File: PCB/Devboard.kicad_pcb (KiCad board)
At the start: 2 copper layers, 133.4 x 151 mm, 602 parts, among them J1 HR911105A_C12074, Q1 IPB180P04P4L-02, Q2 IPB180P04P4L-02, SW1 SW_Push, U1 TVS2201DRBR, U10 TPS62822DLCR, U11 TPS62823DLCR, U12 TPS548A20RVER, U13 TPS7A4700RGWR, U14 TPS3700DSET, U15 TPS54824RNVR, U16 TPS54824RNVR, U17 TPS7A4700RGWR, U18 DW06, U19 TPS61088RHLR, U2 TPD6S300ARUKR, U20 TPS54824RNVR, U21 LM66100DCK, U22 TPS7A4700RGWR, U23 TPS7A4700RGWR, U24 TPS259470ARPWR, U25 TPS54824RNVR, U26 xczu4evfbvb900pkg, U27 RS3112-1.25XSF3, U28 MT25QU256ABA8ESF-0SIT TR, U29 FEMDNN032G-A3A55, U3 STUSB4500QTR, U30 TXS02612RTWR, U31 DP83867IRRGZR, U32 USB3320C-EZK-TR, U34 CP2102N-Axx-xQFN24, U35 TXB0108PW, U36 TCA9548APWR, U37 PCA9306, U38 TPD4E05U06DQA, U4 TPS2121RUXR, U5 TPS259470ARPWR, U6 BQ25895RTWR, U7 BQ27441DRZR-G1A, U8 TPS62130RGTR, U9 XT60, Y1 25 MHz, Y2 25 MHz

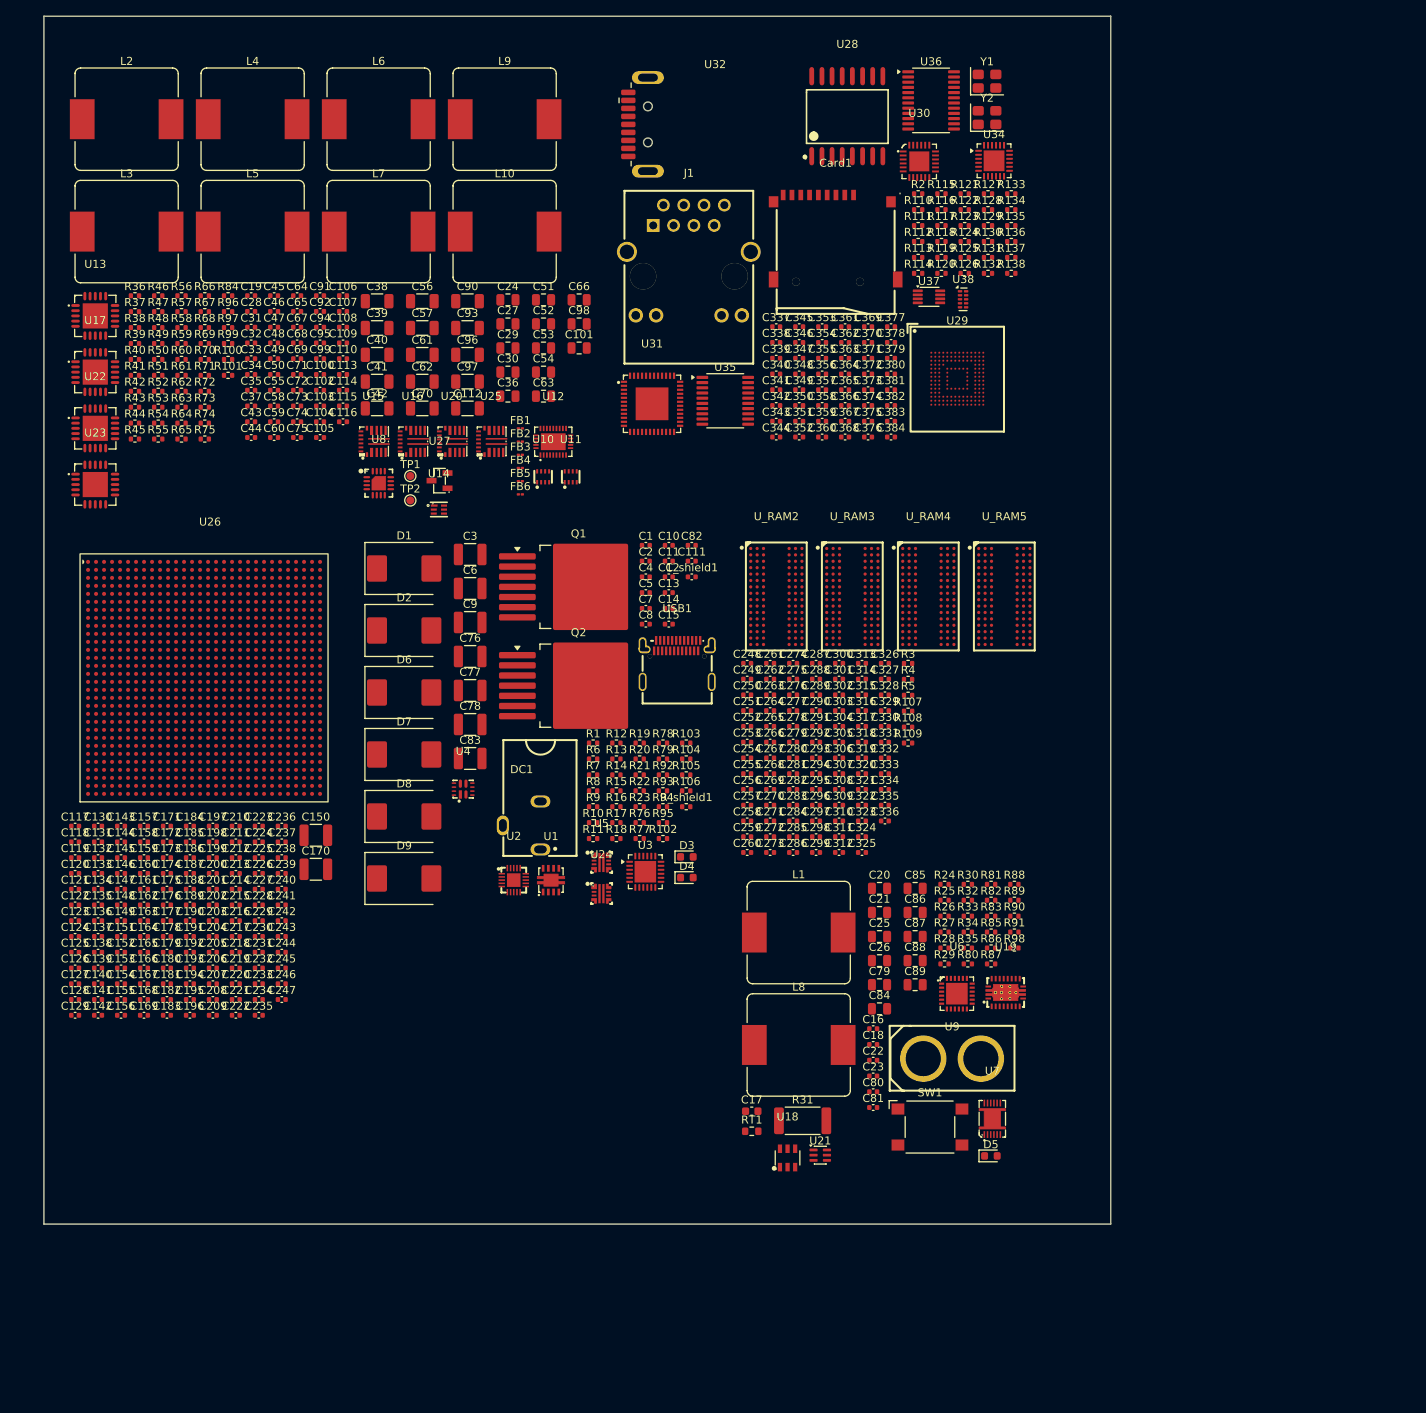
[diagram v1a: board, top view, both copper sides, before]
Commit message: feat: Section 4 Done
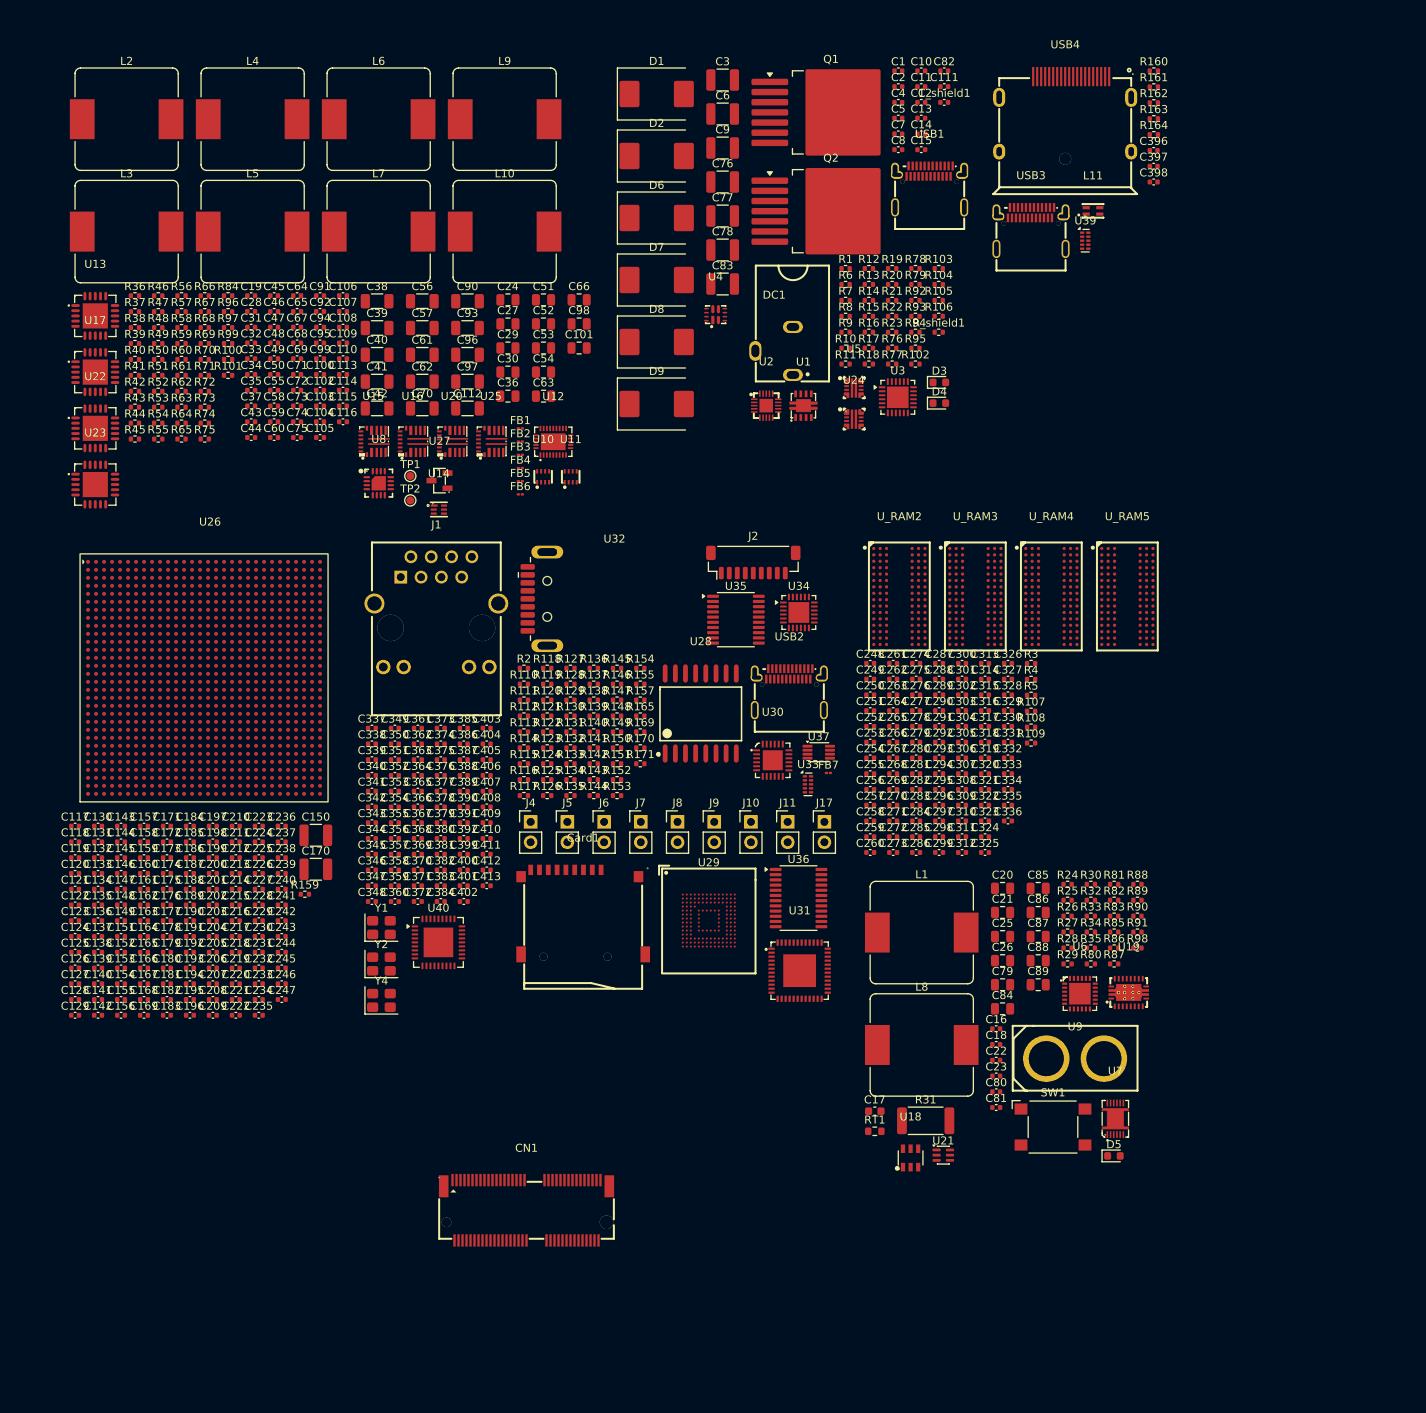
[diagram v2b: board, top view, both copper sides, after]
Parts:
- removed U38: TPD4E05U06DQA, Package_SON:USON-10_2.5x1.0mm_P0.5mm
- added C385: 0.1uF, Capacitor_SMD:C_0402_1005Metric, F.Cu at (49.5, 82.6)
- added C386: 0.1uF, Capacitor_SMD:C_0402_1005Metric, F.Cu at (49.5, 84.6)
- added C387: 1uF, Capacitor_SMD:C_0402_1005Metric, F.Cu at (49.5, 86.6)
- added C388: 0.1uF, Capacitor_SMD:C_0402_1005Metric, F.Cu at (49.5, 88.6)
- added C389: 0.1uF, Capacitor_SMD:C_0402_1005Metric, F.Cu at (49.5, 90.5)
- added C390: 0.1uF, Capacitor_SMD:C_0402_1005Metric, F.Cu at (49.5, 92.5)
- added C391: 0.1uF, Capacitor_SMD:C_0402_1005Metric, F.Cu at (49.5, 94.5)
- added C392: 0.1uF, Capacitor_SMD:C_0402_1005Metric, F.Cu at (49.5, 96.4)
- added C396: 100nF, Capacitor_SMD:C_0402_1005Metric, F.Cu at (135.8, 10.4)
- added C397: 100nF, Capacitor_SMD:C_0402_1005Metric, F.Cu at (135.8, 12.4)
- added C398: 1nF, Capacitor_SMD:C_0402_1005Metric, F.Cu at (135.8, 14.4)
- added C399: 1uF, Capacitor_SMD:C_0402_1005Metric, F.Cu at (49.5, 98.4)
- added C400: 1uF, Capacitor_SMD:C_0402_1005Metric, F.Cu at (49.5, 100.4)
- added C401: 1uF, Capacitor_SMD:C_0402_1005Metric, F.Cu at (49.5, 102.3)
- added C402: 1uF, Capacitor_SMD:C_0402_1005Metric, F.Cu at (49.5, 104.3)
- added C403: 1uF, Capacitor_SMD:C_0402_1005Metric, F.Cu at (52.4, 82.6)
- added C404: 1uF, Capacitor_SMD:C_0402_1005Metric, F.Cu at (52.4, 84.6)
- added C405: 33pF, Capacitor_SMD:C_0402_1005Metric, F.Cu at (52.4, 86.6)
- added C406: 33pF, Capacitor_SMD:C_0402_1005Metric, F.Cu at (52.4, 88.6)
- added C407: 0.1uF, Capacitor_SMD:C_0402_1005Metric, F.Cu at (52.4, 90.5)
- added C408: 0.1uF, Capacitor_SMD:C_0402_1005Metric, F.Cu at (52.4, 92.5)
- added C409: 0.1uF, Capacitor_SMD:C_0402_1005Metric, F.Cu at (52.4, 94.5)
- added C410: 0.1uF, Capacitor_SMD:C_0402_1005Metric, F.Cu at (52.4, 96.4)
- added C411: 1uF, Capacitor_SMD:C_0402_1005Metric, F.Cu at (52.4, 98.4)
- added C412: 0.1uF, Capacitor_SMD:C_0402_1005Metric, F.Cu at (52.4, 100.4)
- added C413: 1nF, Capacitor_SMD:C_0402_1005Metric, F.Cu at (52.4, 102.3)
- added CN1: APCI0120-P001A, Devboard_Footprints:CONN-SMD_APCI0120-P001A, F.Cu at (57.4, 142.9)
- added FB7: BLM18, Inductor_SMD:L_01005_0402Metric, F.Cu at (95.1, 88.2)
- added J10: I2C_7, Connector_PinHeader_2.54mm:PinHeader_1x02_P2.54mm_Vertical, F.Cu at (85.4, 94.4)
- added J11: 3.3V_I2C, Connector_PinHeader_2.54mm:PinHeader_1x02_P2.54mm_Vertical, F.Cu at (90.0, 94.4)
- added J17: I2C_0, Connector_PinHeader_2.54mm:PinHeader_1x02_P2.54mm_Vertical, F.Cu at (94.6, 94.4)
- added J2: USB3_B, Connector_JST:JST_SH_BM09B-SRSS-TB_1x09-1MP_P1.00mm_Vertical, F.Cu at (85.7, 61.9)
- added J4: I2C_1, Connector_PinHeader_2.54mm:PinHeader_1x02_P2.54mm_Vertical, F.Cu at (57.9, 94.4)
- added J5: I2C_2, Connector_PinHeader_2.54mm:PinHeader_1x02_P2.54mm_Vertical, F.Cu at (62.5, 94.4)
- added J6: I2C_3, Connector_PinHeader_2.54mm:PinHeader_1x02_P2.54mm_Vertical, F.Cu at (67.1, 94.4)
- added J7: I2C_4, Connector_PinHeader_2.54mm:PinHeader_1x02_P2.54mm_Vertical, F.Cu at (71.6, 94.4)
- added J8: I2C_5, Connector_PinHeader_2.54mm:PinHeader_1x02_P2.54mm_Vertical, F.Cu at (76.2, 94.4)
- added J9: I2C_6, Connector_PinHeader_2.54mm:PinHeader_1x02_P2.54mm_Vertical, F.Cu at (80.8, 94.4)
- added L11: DLW21HN900SQ2L-CUTTAPE, Devboard_Footprints:FILTER-SMD_4P-L2.0-W1.3-BL_DLW21, F.Cu at (128.2, 18.0)
- added R139: 1kΩ, Resistor_SMD:R_0402_1005Metric, F.Cu at (65.8, 81.1)
- added R140: 8.06kΩ, Resistor_SMD:R_0402_1005Metric, F.Cu at (65.8, 83.1)
- added R141: 10kΩ, Resistor_SMD:R_0402_1005Metric, F.Cu at (65.8, 85.1)
- added R142: 5.1kΩ, Resistor_SMD:R_0402_1005Metric, F.Cu at (65.8, 87.1)
- added R143: 5.1kΩ, Resistor_SMD:R_0402_1005Metric, F.Cu at (65.8, 89.1)
- added R144: 47.5kΩ, Resistor_SMD:R_0402_1005Metric, F.Cu at (65.8, 91.1)
- added R145: 22.1kΩ, Resistor_SMD:R_0402_1005Metric, F.Cu at (68.7, 75.2)
- added R146: 1kΩ, Resistor_SMD:R_0402_1005Metric, F.Cu at (68.7, 77.1)
- added R147: 2.2kΩ, Resistor_SMD:R_0402_1005Metric, F.Cu at (68.7, 79.1)
- added R148: 2.2kΩ, Resistor_SMD:R_0402_1005Metric, F.Cu at (68.7, 81.1)
- added R149: 10kΩ, Resistor_SMD:R_0402_1005Metric, F.Cu at (68.7, 83.1)
- added R150: 2.2kΩ, Resistor_SMD:R_0402_1005Metric, F.Cu at (68.7, 85.1)
- added R151: 2.2kΩ, Resistor_SMD:R_0402_1005Metric, F.Cu at (68.7, 87.1)
- added R152: 2.2kΩ, Resistor_SMD:R_0402_1005Metric, F.Cu at (68.7, 89.1)
- added R153: 2.2kΩ, Resistor_SMD:R_0402_1005Metric, F.Cu at (68.7, 91.1)
- added R154: 200kΩ, Resistor_SMD:R_0402_1005Metric, F.Cu at (71.6, 75.2)
- added R155: 2.2kΩ, Resistor_SMD:R_0402_1005Metric, F.Cu at (71.6, 77.1)
- added R157: 12kΩ, Resistor_SMD:R_0402_1005Metric, F.Cu at (71.6, 79.1)
- added R159: 220Ω, Resistor_SMD:R_0402_1005Metric, F.Cu at (29.7, 103.4)
- added R160: 5.1kΩ, Resistor_SMD:R_0402_1005Metric, F.Cu at (135.8, 0.49)
- added R161: 5.1kΩ, Resistor_SMD:R_0402_1005Metric, F.Cu at (135.8, 2.48)
- added R162: 100kΩ, Resistor_SMD:R_0402_1005Metric, F.Cu at (135.8, 4.47)
- added R163: 100kΩ, Resistor_SMD:R_0402_1005Metric, F.Cu at (135.8, 6.46)
- added R164: 1MΩ, Resistor_SMD:R_0402_1005Metric, F.Cu at (135.8, 8.46)
- added R165: 1MΩ, Resistor_SMD:R_0402_1005Metric, F.Cu at (71.6, 81.1)
- added R169: 100kΩ, Resistor_SMD:R_0402_1005Metric, F.Cu at (71.6, 83.1)
- added R170: 100kΩ, Resistor_SMD:R_0402_1005Metric, F.Cu at (71.6, 85.1)
- added R171: 10kΩ, Resistor_SMD:R_0402_1005Metric, F.Cu at (71.6, 87.1)
- added U33: TPD4E05U06DQA, Package_SON:USON-10_2.5x1.0mm_P0.5mm, F.Cu at (92.5, 89.7)
- added U39: TPD4E05U06DQA, Package_SON:USON-10_2.5x1.0mm_P0.5mm, F.Cu at (127.2, 21.7)
- added U40: USB2514B_Bi, Package_DFN_QFN:QFN-36-1EP_6x6mm_P0.5mm_EP3.7x3.7mm, F.Cu at (46.4, 109.4)
- added USB2: TYPE-C-24P-SMD, Devboard_Footprints:USB-C-SMD_TYPE-C-24P-SMD, F.Cu at (90.2, 77.8)
- added USB3: TYPE-C-24P-SMD, Devboard_Footprints:USB-C-SMD_TYPE-C-24P-SMD, F.Cu at (120.4, 20.1)
- added USB4: 472720001, Devboard_Footprints:CONN-SMD_472720001, F.Cu at (124.7, 5.89)
- added Y4: 26 MHz, Crystal:Crystal_SMD_3225-4Pin_3.2x2.5mm, F.Cu at (39.2, 116.7)
- C379, C380: value 22uF -> 33pF
- U34: value CP2102N-Axx-xQFN24 -> CP2102N-A02-GQFN24
- moved Y1 130.1 mm to (39.2, 107.6)
- moved Y2 130.1 mm to (39.2, 112.1)
- moved U36 101.1 mm to (91.4, 103.9)
- moved Card1 90.1 mm to (64.4, 105.6)
- moved R133 90.1 mm to (62.9, 87.1)
- moved R134 90.1 mm to (62.9, 89.1)
- moved R135 90.1 mm to (62.9, 91.1)
- moved R115 88.3 mm to (57.0, 87.1)
- moved R116 88.3 mm to (57.0, 89.1)
- moved R117 88.3 mm to (57.0, 91.1)
- moved C369 86.7 mm to (43.8, 98.4)
- moved C370 86.7 mm to (43.8, 100.4)
- moved C371 86.7 mm to (43.8, 102.3)
- moved C372 86.7 mm to (43.8, 104.3)
- moved C345 84.9 mm to (38.0, 98.4)
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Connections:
- U26 pad G21: unconnected-(U26-PS_MIO49-PadG21) -> USB3_VBUS_NET
- U26 pad M25: unconnected-(U26-PS_MGTRREF_505-PadM25) -> Net-(U26-PS_MGTRREF_505)
- U32 pad 1: unconnected-(U32-CLKOUT-Pad1) -> USB2_CLK
- U32 pad 2: unconnected-(U32-NXT-Pad2) -> USB2_NXT
- U32 pad 3: unconnected-(U32-DATA0-Pad3) -> USB2_D0
- U32 pad 4: unconnected-(U32-DATA1-Pad4) -> USB2_D1
- U32 pad 5: unconnected-(U32-DATA2-Pad5) -> USB2_D2
- U32 pad 6: unconnected-(U32-DATA3-Pad6) -> USB2_D3
- U32 pad 7: unconnected-(U32-DATA4-Pad7) -> USB2_D4
- U32 pad 9: unconnected-(U32-DATA5-Pad9) -> USB2_D5
- U34 pad 20: unconnected-(U34-RXD-Pad20) -> UART0_RX
- U34 pad 21: unconnected-(U34-TXD-Pad21) -> UART0_TX
- U34 pad 3: unconnected-(U34-D+-Pad3) -> Net-(U33-D2-)
- U34 pad 4: unconnected-(U34-D--Pad4) -> Net-(U33-D2+)
- U34 pad 5: unconnected-(U34-VIO-Pad5) -> +1V8
- U34 pad 6: unconnected-(U34-VDD-Pad6) -> +3V3
- U34 pad 7: unconnected-(U34-VREGIN-Pad7) -> +5V_SYS
- U34 pad 8: VBUS -> Net-(U34-VBUS)
- U34 pad 9: unconnected-(U34-~{RST}-Pad9) -> Net-(U34-~{RST})
- U35 pad 10: unconnected-(U35-OE-Pad10) -> Net-(U35-OE)
- U35 pad 19: unconnected-(U35-V_{CCB}-Pad19) -> +3V3
- U35 pad 2: unconnected-(U35-V_{CCA}-Pad2) -> +1V8
- U36 pad 1: unconnected-(U36-A0-Pad1) -> +1V8
- U36 pad 10: unconnected-(U36-SD3-Pad10) -> I2C_SDA_3
- U36 pad 11: unconnected-(U36-SC3-Pad11) -> I2C_SCL_3
- U36 pad 12: unconnected-(U36-GND-Pad12) -> GND
- U36 pad 13: unconnected-(U36-SD4-Pad13) -> I2C_SDA_4
- U36 pad 14: unconnected-(U36-SC4-Pad14) -> I2C_SCL_4
- U36 pad 15: unconnected-(U36-SD5-Pad15) -> I2C_SDA_5
- U36 pad 16: unconnected-(U36-SC5-Pad16) -> I2C_SCL_5
- U36 pad 17: unconnected-(U36-SD6-Pad17) -> I2C_SDA_6
- U36 pad 18: unconnected-(U36-SC6-Pad18) -> I2C_SCL_6
- U36 pad 19: unconnected-(U36-SD7-Pad19) -> I2C_SDA_7
- U36 pad 2: unconnected-(U36-A1-Pad2) -> +1V8
- U36 pad 20: unconnected-(U36-SC7-Pad20) -> I2C_SCL_7
- U36 pad 21: unconnected-(U36-A2-Pad21) -> +1V8
- U36 pad 22: unconnected-(U36-SCL-Pad22) -> I2C0_SCL
- U36 pad 23: unconnected-(U36-SDA-Pad23) -> I2C0_SDA
- U36 pad 24: unconnected-(U36-VCC-Pad24) -> +1V8
- U36 pad 3: unconnected-(U36-~{RESET}-Pad3) -> Net-(U36-~{RESET})
- U36 pad 4: unconnected-(U36-SD0-Pad4) -> I2C_SDA_0
- U36 pad 5: unconnected-(U36-SC0-Pad5) -> I2C_SCL_0
- U36 pad 6: unconnected-(U36-SD1-Pad6) -> I2C_SDA_1
- U36 pad 7: unconnected-(U36-SC1-Pad7) -> I2C_SCL_1
- U36 pad 8: unconnected-(U36-SD2-Pad8) -> I2C_SDA_2
- U36 pad 9: unconnected-(U36-SC2-Pad9) -> I2C_SCL_2
- U37 pad 2: unconnected-(U37-VREF1-Pad2) -> +1V8
- U37 pad 3: unconnected-(U37-SCL1-Pad3) -> I2C1_SCL
- U37 pad 4: unconnected-(U37-SDA1-Pad4) -> I2C1_SDA
- U37 pad 5: unconnected-(U37-SDA2-Pad5) -> Net-(J11-Pin_1)
- U37 pad 6: unconnected-(U37-SCL2-Pad6) -> Net-(J11-Pin_2)
- U37 pad 7: unconnected-(U37-VREF2-Pad7) -> +3V3
- U37 pad 8: unconnected-(U37-EN-Pad8) -> +3V3
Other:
- board outline removed
